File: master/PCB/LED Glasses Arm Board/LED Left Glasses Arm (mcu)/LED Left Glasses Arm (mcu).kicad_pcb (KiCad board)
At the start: 2 copper layers, 1 part, among them U1 STM32F031E6Yx

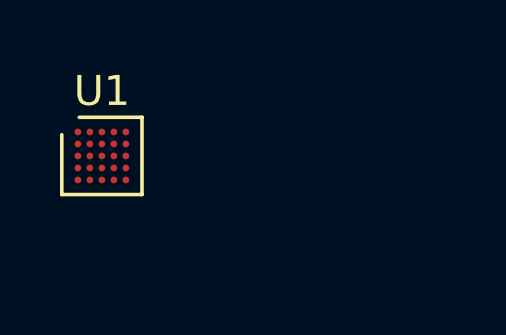
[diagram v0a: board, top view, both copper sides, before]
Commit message: messing around with the MCU
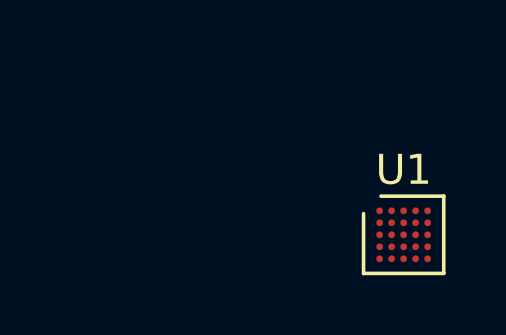
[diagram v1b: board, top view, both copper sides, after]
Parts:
- moved U1 10.4 mm to (130.9, 91.8)
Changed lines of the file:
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@@
   )
   (module Package_CSP:ST_WLCSP-25_Die444 (layer F.Cu)
-    (at 120.8532 89.2048)
+    (at 130.9116 91.8337)
     (descr "WLCSP-25, 5x5 raster, 2.423x2.325mm package, pitch 0.4mm; see section 7.5 of http://www.st.com/resource/en/datasheet/stm32f031k6.pdf")
     (tags "BGA 25 0.4")
